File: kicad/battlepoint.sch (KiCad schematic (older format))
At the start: 32 parts, among them J1 AUDIO, J2 RED_SWITCH, J3 BLU_SWITCH, J4 LED1, J5 LED2, J6 PWR_OPTION, J7 LED3, J8 LED4, P13 BTNS_IN, P14 OLED_OUT, P17 BTNS_OUT, P20 BATT, P40 PWR_SWITCH, P5 SPK, SW1 BTN_UP, SW2 BTN_DWN, SW3 BTN_SEL, U1 DFPLAYER_MINI, U4 L4940

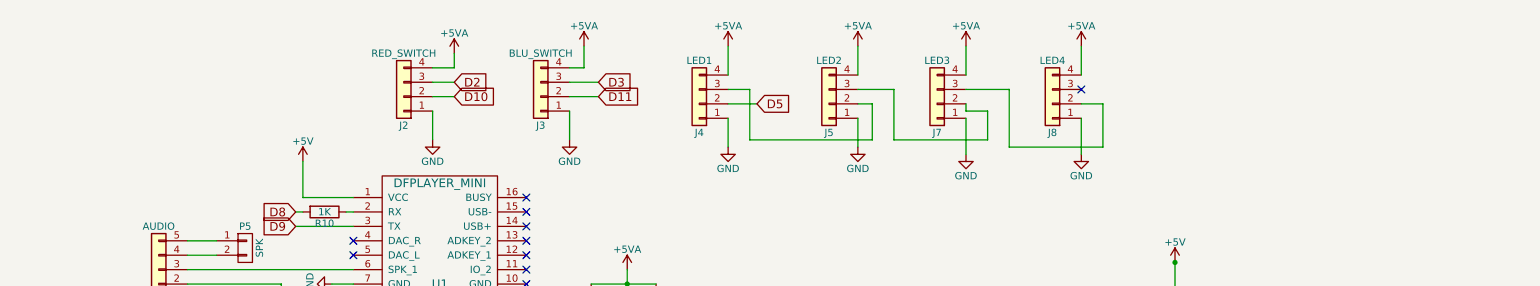
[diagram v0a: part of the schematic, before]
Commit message: finished routing
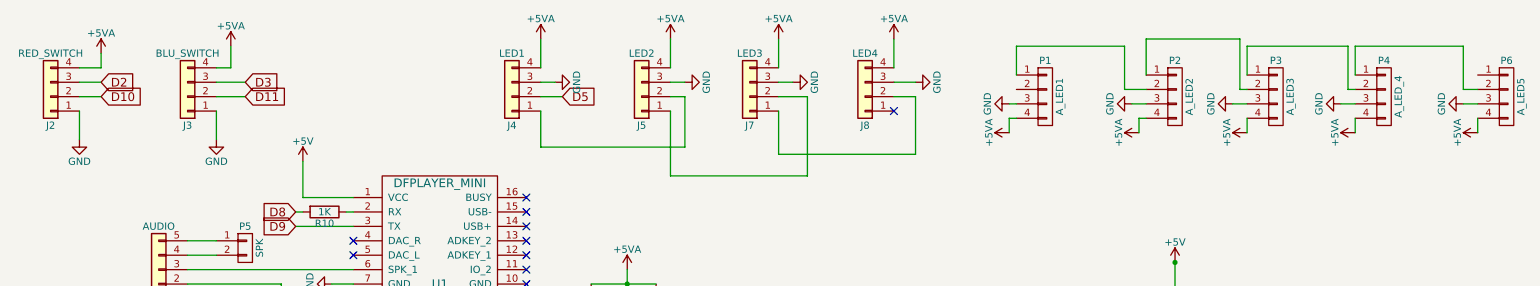
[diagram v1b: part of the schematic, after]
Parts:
- added P1: A_LED1, Connectors_JST:JST_XH_B04B-XH-A_04x2.50mm_Straight, symbol CONN_01X04
- added P2: A_LED2, Connectors_JST:JST_XH_B04B-XH-A_04x2.50mm_Straight, symbol CONN_01X04
- added P3: A_LED3, Connectors_JST:JST_XH_B04B-XH-A_04x2.50mm_Straight, symbol CONN_01X04
- added P4: A_LED_4, Connectors_JST:JST_XH_B04B-XH-A_04x2.50mm_Straight, symbol CONN_01X04
- added P6: A_LED5, Connectors_JST:JST_XH_B04B-XH-A_04x2.50mm_Straight, symbol CONN_01X04
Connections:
- net +5VA: now also P1.4 (P4), P2.4 (P4), P3.4 (P4), P4.4 (P4), P6.4 (P4)
- net GND: now also J4.3 (Pin_3), J5.3 (Pin_3), J7.3 (Pin_3), J8.3 (Pin_3), P1.3 (P3), P2.3 (P3), P3.3 (P3), P4.3 (P3), P6.3 (P3); no longer J4.1 (Pin_1), J5.1 (Pin_1), J7.1 (Pin_1), J8.1 (Pin_1)
- net at J5.2 (Pin_2): now also J4.1 (Pin_1); no longer J4.3 (Pin_3)
- net at J8.2 (Pin_2): now also J7.1 (Pin_1); no longer J7.3 (Pin_3)
- net at J7.2 (Pin_2): now also J5.1 (Pin_1); no longer J5.3 (Pin_3)
- new net: P1.1 (P1), P2.2 (P2)
- new net: P2.1 (P1), P3.2 (P2)
- new net: P3.1 (P1), P4.2 (P2)
- new net: P4.1 (P1), P6.2 (P2)
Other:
- moved on the sheet: J2, J3, J4, J5, J7, J8
